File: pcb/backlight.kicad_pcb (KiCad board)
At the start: 2 copper layers, 100 x 96 mm, 59 parts, among them J3 PJ-002AH, J6 USB_C_Receptacle_USB2.0, U1 AL8860WT, U2 IP2721, U3 AL8860WT, U4 AL8860WT

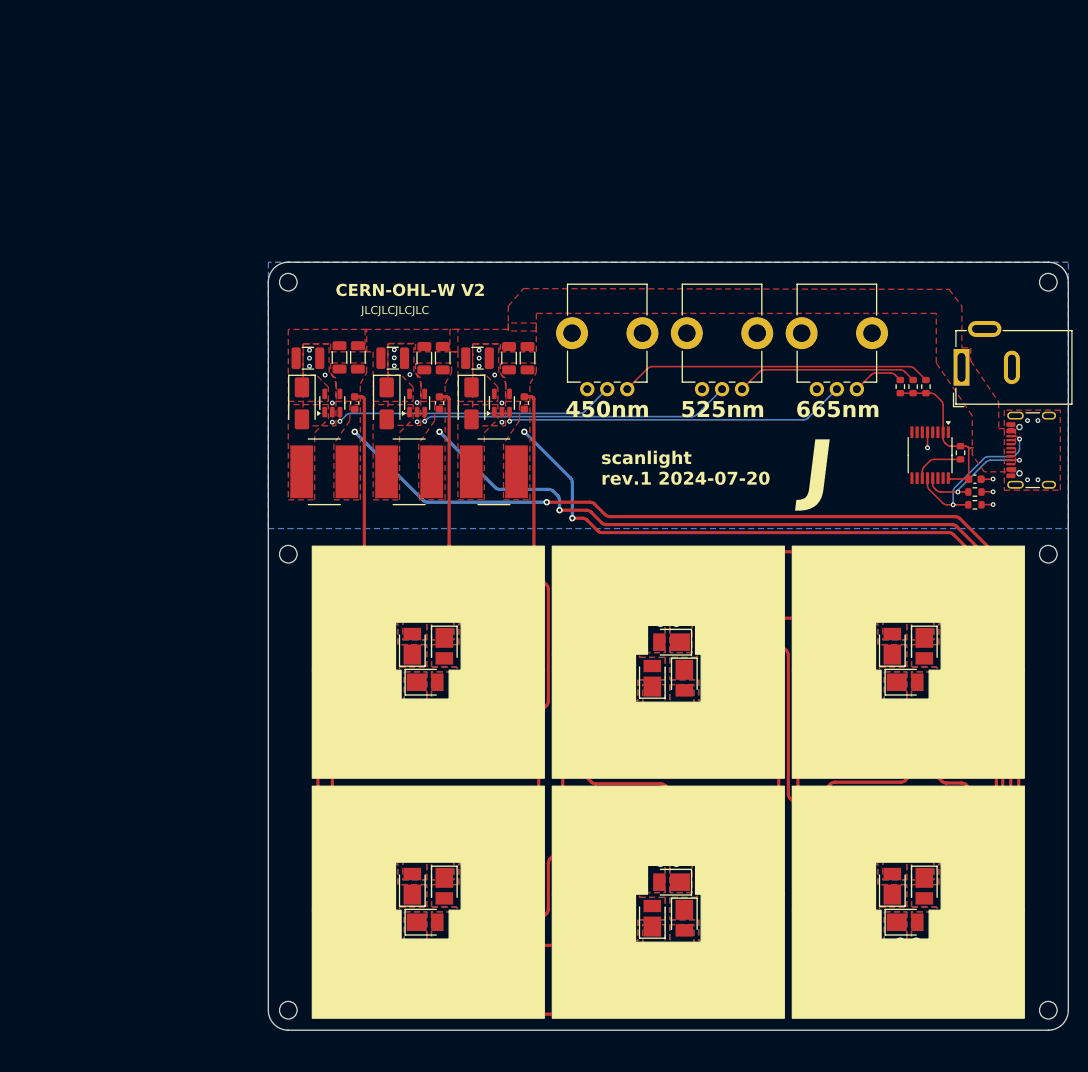
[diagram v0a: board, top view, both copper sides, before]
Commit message: PCB for 4x5 scanlight
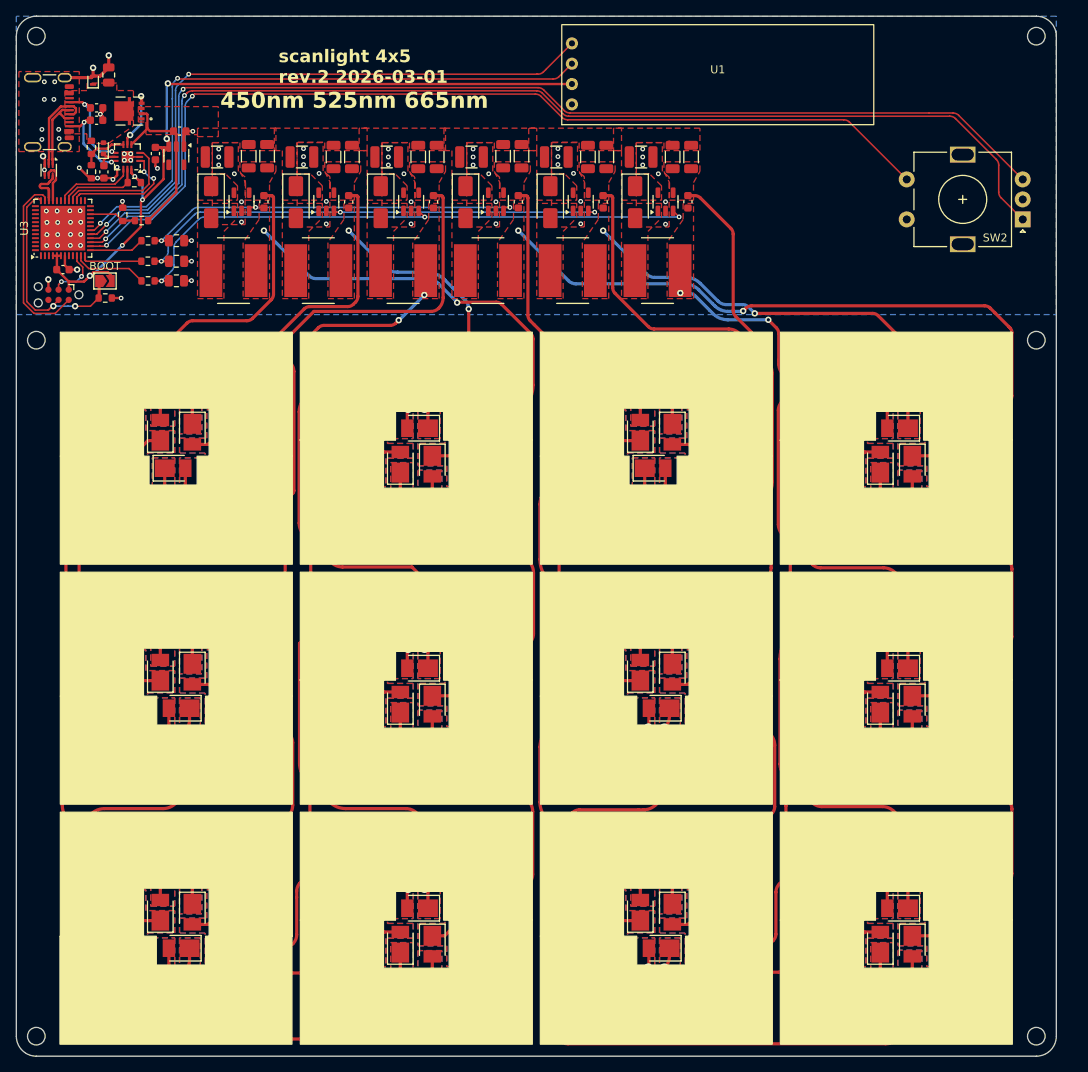
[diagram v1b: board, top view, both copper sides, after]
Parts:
- removed the H1 at (84.5, 145.5)
- removed the H2 at (179.5, 145.5)
- removed J3: PJ-002AH, Connector_BarrelJack:BarrelJack_GCT_DCJ200-10-A_Horizontal
- removed J6: USB_C_Receptacle_USB2.0, Connector_USB:USB_C_Receptacle_GCT_USB4105-xx-A_16P_TopMnt_Horizontal
- removed the R6 at (168.5, 75.8)
- removed RV1, RV2, RV3: 100k, Potentiometer_THT:Potentiometer_Bourns_PTV09A-1_Single_Vertical
- added C1: 330p, Capacitor_SMD:C_0603_1608Metric, F.Cu at (60.5, 34.3)
- added C11: 47n, Capacitor_SMD:C_0805_2012Metric, F.Cu at (70.5, 51.9)
- added C13: 47n, Capacitor_SMD:C_0805_2012Metric, F.Cu at (70.5, 49.3)
- added C14: 1u, Capacitor_SMD:C_0603_1608Metric, F.Cu at (113.2, 44.5)
- added C16: 10u, Capacitor_SMD:C_1210_3225Metric, F.Cu at (107.4, 38.9)
- added C19: 1u, Capacitor_SMD:C_0603_1608Metric, F.Cu at (134.4, 44.5)
- added C2: 330p, Capacitor_SMD:C_0603_1608Metric, F.Cu at (60.5, 32.7)
- added C20: 10u, Capacitor_SMD:C_1210_3225Metric, F.Cu at (118.0, 38.9)
- added C21: 10u, Capacitor_SMD:C_1210_3225Metric, F.Cu at (128.6, 38.9)
- added C22: 1u, Capacitor_SMD:C_0603_1608Metric, F.Cu at (123.8, 44.5)
- added C3: 4.7u, Capacitor_SMD:C_0805_2012Metric, F.Cu at (62.0, 28.6)
- added C5: 0.1u, Capacitor_SMD:C_0603_1608Metric, F.Cu at (61.4, 40.7)
- added C6: 0.1u, Capacitor_SMD:C_0603_1608Metric, F.Cu at (56.3, 52.9)
- added C7: 47n, Capacitor_SMD:C_0805_2012Metric, F.Cu at (70.5, 54.3)
- added C8: 1u, Capacitor_SMD:C_0603_1608Metric, F.Cu at (67.9, 38.4)
- added D1: BAT54K, Diode_SMD:D_SOD-523, F.Cu at (61.4, 37.8)
- added D12: red, LED_SMD:LED_PLCC_2835_Handsoldering_Reverse, F.Cu at (72.5, 133.2)
- added D18: green, LED_SMD:LED_PLCC_2835_Handsoldering, F.Cu at (160.9, 72.8)
- added D19: blue, LED_SMD:LED_PLCC_2835_Handsoldering, F.Cu at (162.5, 77.2)
- added D2: ESDA25P35, Diode_SMD:ST_QFN-2L_1.6x1.0mm, F.Cu at (60.1, 29.2)
- added D20: red, LED_SMD:LED_PLCC_2835_Handsoldering_Reverse, F.Cu at (158.5, 77.2)
- added D30: blue, LED_SMD:LED_PLCC_2835_Handsoldering, F.Cu at (162.5, 107.2)
- added D31: red, LED_SMD:LED_PLCC_2835_Handsoldering_Reverse, F.Cu at (158.5, 107.2)
- added D32: green, LED_SMD:LED_PLCC_2835_Handsoldering, F.Cu at (160.9, 102.8)
- added D33: green, LED_SMD:LED_PLCC_2835_Handsoldering, F.Cu at (71.1, 137.8)
- added D35: blue, LED_SMD:LED_PLCC_2835_Handsoldering, F.Cu at (68.5, 133.2)
- added D36: blue, LED_SMD:LED_PLCC_2835_Handsoldering, F.Cu at (102.5, 137.2)
- added D37: green, LED_SMD:LED_PLCC_2835_Handsoldering, F.Cu at (100.9, 132.8)
- added D38: red, LED_SMD:LED_PLCC_2835_Handsoldering_Reverse, F.Cu at (98.5, 137.2)
- added D39: green, LED_SMD:LED_PLCC_2835_Handsoldering, F.Cu at (131.1, 137.8)
- added D40: blue, LED_SMD:LED_PLCC_2835_Handsoldering, F.Cu at (128.5, 133.2)
- added D41: red, LED_SMD:LED_PLCC_2835_Handsoldering_Reverse, F.Cu at (132.5, 133.2)
- added D42: blue, LED_SMD:LED_PLCC_2835_Handsoldering, F.Cu at (162.5, 137.2)
- added D43: green, LED_SMD:LED_PLCC_2835_Handsoldering, F.Cu at (160.9, 132.8)
- added D44: red, LED_SMD:LED_PLCC_2835_Handsoldering_Reverse, F.Cu at (158.5, 137.2)
- added D6: B240A, Diode_SMD:D_SMA, F.Cu at (106.7, 44.5)
- added D7: B240A, Diode_SMD:D_SMA, F.Cu at (127.8, 44.5)
- added D8: B240A, Diode_SMD:D_SMA, F.Cu at (117.2, 44.5)
- added H5: MountingHole, MountingHole:MountingHole_2.2mm_M2_Mask_5mm, F.Cu at (53.0, 148.8)
- added H6: MountingHole, MountingHole:MountingHole_2.2mm_M2_Mask_5mm, F.Cu at (178.0, 148.8)
- added J1: UJ20-C-H-G-SMT-P16-TR, Custom:USB_C_Receptacle_UJ20-C-H-G-SMT-P16-TR, F.Cu at (53.4, 33.2)
- added J2: SWD_TC2030, Connector:Tag-Connect_TC2030-IDC-NL_2x03_P1.27mm_Vertical, F.Cu at (55.8, 56.1)
- added L4: 100u, Inductor_SMD:L_Bourns_SRN8040TA, F.Cu at (109.5, 53.0)
- added L5: 100u, Inductor_SMD:L_Bourns_SRN8040TA, F.Cu at (130.7, 53.0)
- added L6: 100u, Inductor_SMD:L_Bourns_SRN8040TA, F.Cu at (120.0, 53.0)
- added Q1: STL11N3LLH6, Custom:POWERFLAT-3p3X3p3_STM, F.Cu at (64.6, 33.1)
- added R1: 10k, Resistor_SMD:R_0603_1608Metric, F.Cu at (59.9, 37.6)
- added R10: 10k, Resistor_SMD:R_0603_1608Metric, F.Cu at (65.2, 42.0)
- added R12: 845m, Resistor_SMD:R_1206_3216Metric, F.Cu at (111.3, 38.8)
- added R17: 845m, Resistor_SMD:R_1206_3216Metric, F.Cu at (113.7, 38.8)
- added R18: 845m, Resistor_SMD:R_1206_3216Metric, F.Cu at (124.3, 38.9)
- added R19: 845m, Resistor_SMD:R_1206_3216Metric, F.Cu at (122.0, 38.9)
- added R20: 845m, Resistor_SMD:R_1206_3216Metric, F.Cu at (134.8, 38.9)
- added R21: 845m, Resistor_SMD:R_1206_3216Metric, F.Cu at (132.5, 38.9)
- added R4: 200k, Resistor_SMD:R_0603_1608Metric, F.Cu at (66.2, 46.8)
- added R9: 40.2k, Resistor_SMD:R_0603_1608Metric, F.Cu at (63.8, 46.0)
- added SW1: BOOT, Jumper:SolderJumper-2_P1.3mm_Open_TrianglePad1.0x1.5mm, F.Cu at (61.6, 54.4)
- added SW2: RotaryEncoder_Switch_MP, Rotary_Encoder:RotaryEncoder_Alps_EC11E-Switch_Vertical_H20mm, F.Cu at (176.3, 46.6)
- added U1: 0.91 Inch OLED, Display:0.91_Inch_OLED, F.Cu at (138.2, 28.4)
- added U10: AL8860WT, Package_TO_SOT_SMD:TSOT-23-5, F.Cu at (121.0, 44.5)
- added U11: AL8860WT, Package_TO_SOT_SMD:TSOT-23-5, F.Cu at (131.7, 44.5)
- added U3: STM32G0B1CBUx, Package_DFN_QFN:QFN-48-1EP_7x7mm_P0.5mm_EP5.6x5.6mm, F.Cu at (56.3, 47.8)
- added U4: TCPP01_M12, Custom:QFN-12-1EP_3x3mm_P0.50mm_EP1.45x1.45mm, F.Cu at (64.4, 38.8)
- added U6: ST732M33R, Package_TO_SOT_SMD:TSOT-23-5, F.Cu at (70.5, 38.7)
- added U8: AL8860WT, Package_TO_SOT_SMD:TSOT-23-5, F.Cu at (110.5, 44.5)
- D11: renamed from D1; value deep blue -> blue
- D14: renamed from D4; value deep blue -> blue
- D15: renamed from D20; value deep red -> red; footprint LED_SMD:LED_PLCC_2835_Handsoldering -> LED_SMD:LED_PLCC_2835_Handsoldering_Reverse
- D16: renamed from D5; value deep blue -> blue
- D23: renamed from D2; value deep blue -> blue
- D24: renamed from D19; value deep red -> red; footprint LED_SMD:LED_PLCC_2835_Handsoldering -> LED_SMD:LED_PLCC_2835_Handsoldering_Reverse
- D26: renamed from D3; value deep blue -> blue
- D27: renamed from D21; value deep red -> red; footprint LED_SMD:LED_PLCC_2835_Handsoldering -> LED_SMD:LED_PLCC_2835_Handsoldering_Reverse
- D28: renamed from D6; value deep blue -> blue
- D34: renamed from D18; value deep red -> red; footprint LED_SMD:LED_PLCC_2835_Handsoldering -> LED_SMD:LED_PLCC_2835_Handsoldering_Reverse
- D5: renamed from D16; value deep red -> red; footprint LED_SMD:LED_PLCC_2835_Handsoldering -> LED_SMD:LED_PLCC_2835_Handsoldering_Reverse
- D9: renamed from D17; value deep red -> red; footprint LED_SMD:LED_PLCC_2835_Handsoldering -> LED_SMD:LED_PLCC_2835_Handsoldering_Reverse
- H1: renamed from H5; footprint Custom:MountingHole_2.2mm_M2_Mask_5mm -> MountingHole:MountingHole_2.2mm_M2_Mask_5mm
- H2: renamed from H6; footprint Custom:MountingHole_2.2mm_M2_Mask_5mm -> MountingHole:MountingHole_2.2mm_M2_Mask_5mm
- H3, H4: footprint Custom:MountingHole_2.2mm_M2_Mask_5mm -> MountingHole:MountingHole_2.2mm_M2_Mask_5mm
- R11: renamed from R1; value 1.4 -> 845m
- R13: renamed from R9; value 1.4 -> 845m
- R14: renamed from R11; value 1.4 -> 845m
- R15: renamed from R4; value 1.4 -> 845m
- R16: renamed from R12; value 1.4 -> 845m
- R2: value 649k -> 100k
- R3: value 649k -> 620
- R5: value 649k -> 4.7k
- R6: renamed from R10; value 1.4 -> 845m
- R7, R8: value 5.1k -> 4.7k
- SYM1: renamed from SYM101; footprint Custom:hot-surface_1x -> Symbol:HOT
- U2: value IP2721 -> ECMF02-2AMX6; footprint Package_SO:TSSOP-16_4.4x5mm_P0.65mm -> Package_DFN_QFN:ST_UQFN-6L_1.5x1.7mm_P0.5mm
- moved U2 115.8 mm to (54.5, 40.5)
- moved C4 108.5 mm to (70.9, 35.6)
- moved R8 108.5 mm to (67.0, 49.3), turned to 180 degrees
- moved R7 107.3 mm to (66.9, 51.9), turned to 180 degrees
- moved R3 106.2 mm to (59.9, 40.7), turned to -90 degrees
- moved R2 103.2 mm to (61.6, 56.5), turned to 0 degrees
- moved R5 95.0 mm to (67.0, 54.3), turned to 180 degrees
- moved H1 44.0 mm to (53.0, 23.8)
- moved D10 41.3 mm to (70.1, 77.8)
- moved D11 41.3 mm to (68.5, 73.2)
- moved D13 41.3 mm to (100.9, 72.7)
- moved D14 41.3 mm to (102.5, 77.2)
- moved D15 41.3 mm to (132.5, 73.2)
- moved D16 41.3 mm to (128.5, 73.2)
- moved D17 41.3 mm to (130.1, 77.8)
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- renumbered C1 to C10, C3 to C12, C5 to C15, C6 to C17, C7 to C18, C2 to C9, D9 to D10, D12 to D13, D13 to D17, D15 to D21, D10 to D22, D11 to D25, D14 to D29, D7 to D3, D8 to D4, U1 to U5, U3 to U7, U4 to U9
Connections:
- net Net-(D1-A) renamed /LED_Blue1/Set
- net Net-(D1-K) renamed /LED_Blue1/D0
- net Net-(D10-A) renamed /LED_Green1/D0
- net Net-(D11-K) renamed /LED_Green1/D4
- net Net-(D13-K) renamed /LED_Green2/D0
- net Net-(D15-A) renamed /LED_Red1/SW
- net Net-(D3-K) renamed /LED_Blue1/D4
- net Net-(D5-K) renamed /LED_Blue2/D0
- net Net-(D7-A) renamed /LED_Blue1/SW
- net Net-(D8-A) renamed /LED_Green1/SW
- net Net-(D9-A) renamed /LED_Green1/Set
- C10 pad 1: +20V -> VBUS
- C12 pad 1: +20V -> VBUS
- C15 pad 2: Net-(D14-K) -> /LED_Green1/LC
- C17 pad 1: +20V -> VBUS
- C18 pad 1: Net-(D16-A) -> /LED_Red1/Set
- C18 pad 2: Net-(D21-K) -> /LED_Red1/LC
- C4 pad 2: +20V -> VBUS
- C9 pad 2: Net-(D6-K) -> /LED_Blue1/LC
- D13 pad 1: Net-(D12-K) -> /LED_Green1/LC
- D14 pad 1: Net-(D4-K) -> /LED_Blue1/LC
- D15 pad 1: Net-(D19-K) -> /LED_Red2/D0
- D15 pad 2: Net-(D20-K) -> /LED_Red2/Set
- D16 pad 2: Net-(D4-K) -> /LED_Blue2/Set
- D17 pad 2: Net-(D12-K) -> /LED_Green2/Set
- D21 pad 1: +20V -> VBUS
- D22 pad 1: Net-(D10-K) -> /LED_Green1/D1
- D23 pad 1: Net-(D2-K) -> /LED_Blue1/D1
- D24 pad 1: Net-(D18-K) -> /LED_Red1/LC
- D24 pad 2: Net-(D19-K) -> /LED_Red1/D4
- D25 pad 2: Net-(D10-K) -> /LED_Green1/D3
- D26 pad 2: Net-(D2-K) -> /LED_Blue1/D3
- D27 pad 1: Net-(D20-K) -> /LED_Red2/D1
- D27 pad 2: Net-(D21-K) -> /LED_Red2/D0
- D28 pad 1: Net-(D6-K) -> /LED_Blue2/D1
- D29 pad 1: Net-(D14-K) -> /LED_Green2/D1
- D3 pad 1: +20V -> VBUS
- D34 pad 1: Net-(D17-K) -> /LED_Red1/D4
- D34 pad 2: Net-(D18-K) -> /LED_Red1/D3
- D4 pad 1: +20V -> VBUS
- D5 pad 1: Net-(D16-A) -> /LED_Red1/D0
- D5 pad 2: Net-(D16-K) -> /LED_Red1/Set
- D9 pad 1: Net-(D16-K) -> /LED_Red1/D1
- D9 pad 2: Net-(D17-K) -> /LED_Red1/D0
- L1 pad 1: Net-(D6-K) -> /LED_Blue1/LC
- L2 pad 1: Net-(D14-K) -> /LED_Green1/LC
- L3 pad 1: Net-(D21-K) -> /LED_Red1/LC
- R11 pad 1: +20V -> VBUS
- R13 pad 1: +20V -> VBUS
- R13 pad 2: Net-(D16-A) -> /LED_Red1/Set
- R14 pad 1: +20V -> VBUS
- R14 pad 2: Net-(D16-A) -> /LED_Red1/Set
- R15 pad 1: +20V -> VBUS
- R16 pad 1: +20V -> VBUS
- R2 pad 1: +20V -> /SWCLK
- R2 pad 2: Net-(R2-Pad2) -> GND
- R3 pad 1: +20V -> /Power/VBUS_CTRL
- R3 pad 2: Net-(R3-Pad2) -> GND
- R5 pad 1: +20V -> /CTRL_R
- R5 pad 2: Net-(R5-Pad2) -> /PWM_R
- R6 pad 1: +20V -> VBUS
- R7 pad 1: Net-(J6-CC1) -> /CTRL_G
- R7 pad 2: GND -> /PWM_G
- R8 pad 1: Net-(J6-CC2) -> /CTRL_B
- R8 pad 2: GND -> /PWM_B
- U2 pad 1: unconnected-(U2-VBUSG-Pad1) -> /Power/D0+
- U2 pad 2: +20V -> /Power/D0-
- U2 pad 3: unconnected-(U2-NC-Pad3) -> GND
- U2 pad 4: unconnected-(U2-NC-Pad4) -> GND
- U2 pad 5: GND -> /D-
- U2 pad 6: unconnected-(U2-NC-Pad6) -> /D+
- U5 pad 3: Net-(U1-CTRL) -> /CTRL_B
- U5 pad 5: +20V -> VBUS
- U7 pad 3: Net-(U3-CTRL) -> /CTRL_G
- U7 pad 5: +20V -> VBUS
- U9 pad 3: Net-(U4-CTRL) -> /CTRL_R
- U9 pad 4: Net-(D16-A) -> /LED_Red1/Set
- U9 pad 5: +20V -> VBUS
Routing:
- net Net-(D6-K): track 180.6 -> 0.00 mm, vias 12 -> 0
- net Net-(D14-K): track 146.8 -> 0.00 mm, vias 12 -> 0
- net /R_Q: track 0.00 -> 139.5 mm, vias 0 -> 2
- net /R_I: track 0.00 -> 135.5 mm, vias 0 -> 2
- net /R_SW: track 0.00 -> 120.3 mm, vias 0 -> 2
- net Net-(D21-K): track 106.2 -> 0.00 mm, vias 13 -> 0
- net +3.3V: track 0.00 -> 100.0 mm, vias 0 -> 6
- net /LED_Blue2/LC: track 0.00 -> 80.7 mm, vias 0 -> 13
- net /SDA: track 0.00 -> 77.4 mm, vias 0 -> 2
- net /SCL: track 0.00 -> 76.0 mm, vias 0 -> 2
- net /CTRL_R: track 0.00 -> 73.6 mm, vias 0 -> 3
- net /LED_Blue2/D2: track 0.00 -> 62.3 mm, vias 0 -> 22
- net /LED_Blue1/D2: track 0.00 -> 61.8 mm, vias 0 -> 22
- net /CTRL_G: track 0.00 -> 61.3 mm, vias 0 -> 3
- net /LED_Green2/Set: track 0.00 -> 57.3 mm, vias 0 -> 12
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- added copper zone on B.Cu, net /LED_Blue1/D1
- added copper zone on F.Cu, net /LED_Blue1/D1
- added copper zone on B.Cu, net /LED_Blue1/D2
- added copper zone on F.Cu, net /LED_Blue1/D2
- added copper zone on B.Cu, net /LED_Blue1/D3
- added copper zone on F.Cu, net /LED_Blue1/D3
- added copper zone on B.Cu, net /LED_Blue1/LC
- added copper zone on F.Cu, net /LED_Blue1/LC
- added copper zone on B.Cu, net /LED_Blue2/D1
- added copper zone on F.Cu, net /LED_Blue2/D1
- added copper zone on B.Cu, net /LED_Blue2/D2
- added copper zone on F.Cu, net /LED_Blue2/D2
- added copper zone on B.Cu, net /LED_Blue2/D3
- added copper zone on F.Cu, net /LED_Blue2/D3
- added copper zone on B.Cu, net /LED_Blue2/D4
- added copper zone on F.Cu, net /LED_Blue2/D4
- added copper zone on B.Cu, net /LED_Blue2/LC
- added copper zone on F.Cu, net /LED_Blue2/LC
- added copper zone on F.Cu, net /LED_Blue2/SW
- added copper zone on B.Cu, net /LED_Blue2/Set
- added copper zone on F.Cu, net /LED_Blue2/Set
- added copper zone on B.Cu, net /LED_Green1/D1
- added copper zone on F.Cu, net /LED_Green1/D1
- added copper zone on B.Cu, net /LED_Green1/D2
- added copper zone on F.Cu, net /LED_Green1/D2
- added copper zone on B.Cu, net /LED_Green1/D3
- added copper zone on F.Cu, net /LED_Green1/D3
- added copper zone on B.Cu, net /LED_Green1/LC
- added copper zone on F.Cu, net /LED_Green1/LC
- added copper zone on B.Cu, net /LED_Green2/D1
- added copper zone on F.Cu, net /LED_Green2/D1
- added copper zone on B.Cu, net /LED_Green2/D2
- added copper zone on F.Cu, net /LED_Green2/D2
- added copper zone on B.Cu, net /LED_Green2/D3
- added copper zone on F.Cu, net /LED_Green2/D3
- added copper zone on B.Cu, net /LED_Green2/D4
- added copper zone on F.Cu, net /LED_Green2/D4
- added copper zone on B.Cu, net /LED_Green2/LC
- added copper zone on F.Cu, net /LED_Green2/LC
- added copper zone on F.Cu, net /LED_Green2/SW
- added copper zone on B.Cu, net /LED_Green2/Set
- added copper zone on F.Cu, net /LED_Green2/Set
- added copper zone on B.Cu, net /LED_Red1/D0
- added copper zone on F.Cu, net /LED_Red1/D0
- added copper zone on B.Cu, net /LED_Red1/D1
- added copper zone on F.Cu, net /LED_Red1/D1
- added copper zone on B.Cu, net /LED_Red1/D2
- added copper zone on F.Cu, net /LED_Red1/D2
- added copper zone on B.Cu, net /LED_Red1/D3
- added copper zone on F.Cu, net /LED_Red1/D3
- added copper zone on B.Cu, net /LED_Red1/D4
- added copper zone on F.Cu, net /LED_Red1/D4
- added copper zone on B.Cu, net /LED_Red1/LC
- added copper zone on F.Cu, net /LED_Red1/LC
- added copper zone on B.Cu, net /LED_Red1/Set
- added copper zone on F.Cu, net /LED_Red1/Set
- added copper zone on B.Cu, net /LED_Red2/D0
- added copper zone on F.Cu, net /LED_Red2/D0
- added copper zone on B.Cu, net /LED_Red2/D1
- added copper zone on F.Cu, net /LED_Red2/D1
- added copper zone on B.Cu, net /LED_Red2/D2
- added copper zone on F.Cu, net /LED_Red2/D2
- added copper zone on B.Cu, net /LED_Red2/D3
- added copper zone on F.Cu, net /LED_Red2/D3
- added copper zone on B.Cu, net /LED_Red2/D4
- added copper zone on F.Cu, net /LED_Red2/D4
- added copper zone on B.Cu, net /LED_Red2/LC
- added copper zone on F.Cu, net /LED_Red2/LC
- added copper zone on F.Cu, net /LED_Red2/SW
- added copper zone on B.Cu, net /LED_Red2/Set
- added copper zone on F.Cu, net /LED_Red2/Set
- added copper zone on F.Cu, net VBUS
- added copper zone on F.Cu, net VDC
- removed copper zone on F.Cu, net +20V
- removed copper zone on B.Cu, net Net-(D10-K)
- removed copper zone on F.Cu, net Net-(D10-K)
- removed copper zone on B.Cu, net Net-(D12-K)
- removed copper zone on F.Cu, net Net-(D12-K)
- removed copper zone on B.Cu, net Net-(D14-K)
- removed copper zone on F.Cu, net Net-(D14-K)
- removed copper zone on B.Cu, net Net-(D16-A)
- removed copper zone on F.Cu, net Net-(D16-A)
- removed copper zone on B.Cu, net Net-(D16-K)
- removed copper zone on F.Cu, net Net-(D16-K)
- removed copper zone on B.Cu, net Net-(D17-K)
- removed copper zone on F.Cu, net Net-(D17-K)
- removed copper zone on B.Cu, net Net-(D18-K)
- removed copper zone on F.Cu, net Net-(D18-K)
- removed copper zone on B.Cu, net Net-(D19-K)
- removed copper zone on F.Cu, net Net-(D19-K)
- removed copper zone on B.Cu, net Net-(D2-K)
- removed copper zone on F.Cu, net Net-(D2-K)
- removed copper zone on B.Cu, net Net-(D20-K)
- removed copper zone on F.Cu, net Net-(D20-K)
- removed copper zone on B.Cu, net Net-(D21-K)
- removed copper zone on F.Cu, net Net-(D21-K)
- removed copper zone on B.Cu, net Net-(D4-K)
- removed copper zone on F.Cu, net Net-(D4-K)
- removed copper zone on B.Cu, net Net-(D6-K)
- removed copper zone on F.Cu, net Net-(D6-K)
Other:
- board size 100 x 96 mm -> 130 x 130 mm
- board text added: "1u"
- board text added: "450nm 525nm 665nm"
- board text added: "470"
- board text added: "PCB specifications: - 2 copper layers - size: 130.0 x 130.0 mm - thickness: 1.6 mm - material: FR4 TG-140+ - min track width/spacing: 0.2 mm - min hole size: 0.3 mm - min annular ring size: 0.15mm - soldermask: black - silkscreen: white - finish: Lead Free HASL - copper: 1 oz"
- board text added: "USB PD 20V"
- board text added: "William Buxton CERN-OHL-W V2"
- board text added: "scanlight 4x5 rev.2 2026-03-01"
- board text removed: "450nm"
- board text removed: "525nm"
- board text removed: "665nm"
- board text removed: "CERN-OHL-W V2"
- board text removed: "INPUT: 19-24V DC 500mA USB PD 20V only"
- board text removed: "J"
- board text removed: "JLCJLCJLCJLC"
- board text removed: "PCB specifications: - 2 copper layers - size: 100.0 x 96.0 mm - thickness: 1.6 mm - material: FR4 TG-140+ - min track width/spacing: 0.2 mm - min hole size: 0.3 mm - min annular ring size: 0.15mm - soldermask: black - silkscreen: white - finish: HASL - copper: 1 oz"
- board text removed: "scanlight rev.1 2024-07-20"
